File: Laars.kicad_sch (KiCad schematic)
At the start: 12 parts, among them Q1 NMOS, Q2 NPN

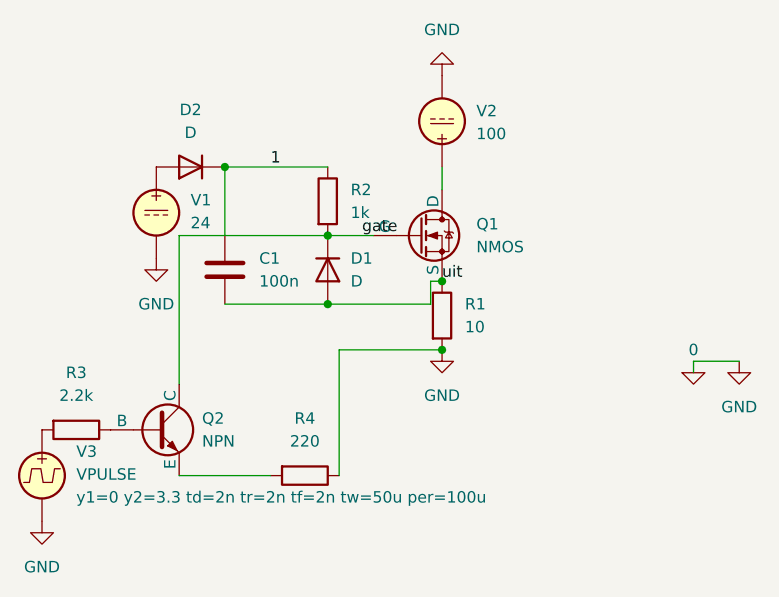
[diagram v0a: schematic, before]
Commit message: V4
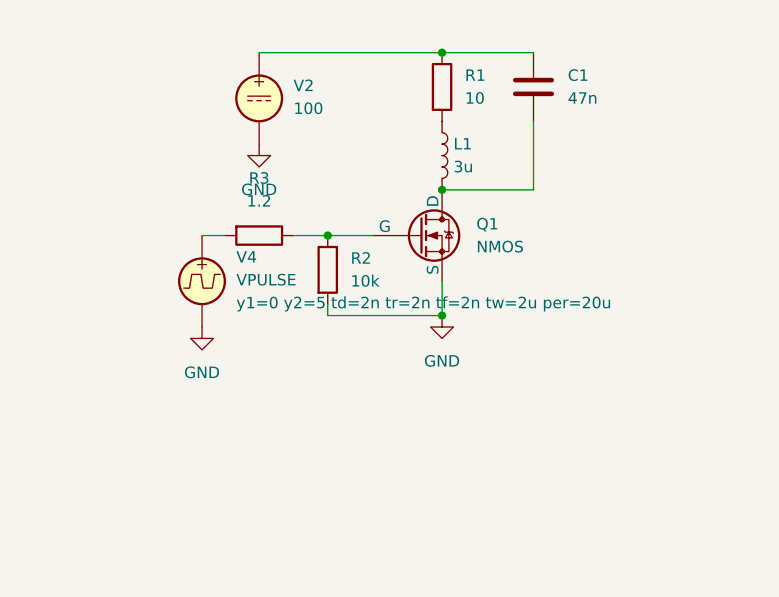
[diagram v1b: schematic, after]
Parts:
- removed D1, D2: D, symbol Device:D
- removed Q2: NPN, symbol Simulation_SPICE:NPN
- removed R4: 220, symbol Device:R
- removed V1: 24, symbol Simulation_SPICE:VDC
- removed V3: VPULSE, symbol Simulation_SPICE:VPULSE
- added L1: 3u, symbol Device:L
- added V4: VPULSE, symbol Simulation_SPICE:VPULSE
- C1: value 100n -> 47n
- R2: value 1k -> 10k
- R3: value 2.2k -> 1.2
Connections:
- net at V2.1: now also C1.1, R1.1; no longer Q1.1 (D)
- net at R3.2: now also V4.1
- net at R3.1: now also Q1.2 (G), R2.1
- net 0: no longer names the net of R1.2
- net 0: now also L1.1; no longer V2.2
- removed net 1: C1.1, R2.1
- net gate renamed GND
- net GND: now also Q1.3 (S), V2.2, V4.2; no longer Q1.2 (G)
- removed net uit: C1.2, Q1.3 (S), R1.1
- new net: C1.2, L1.2, Q1.1 (D)
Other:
- moved on the sheet: V2
